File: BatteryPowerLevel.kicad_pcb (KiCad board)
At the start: 2 copper layers, 22.2 x 23.9 mm, 30 parts, among them J1 Conn_01x02_Male, SW1 SW_Push

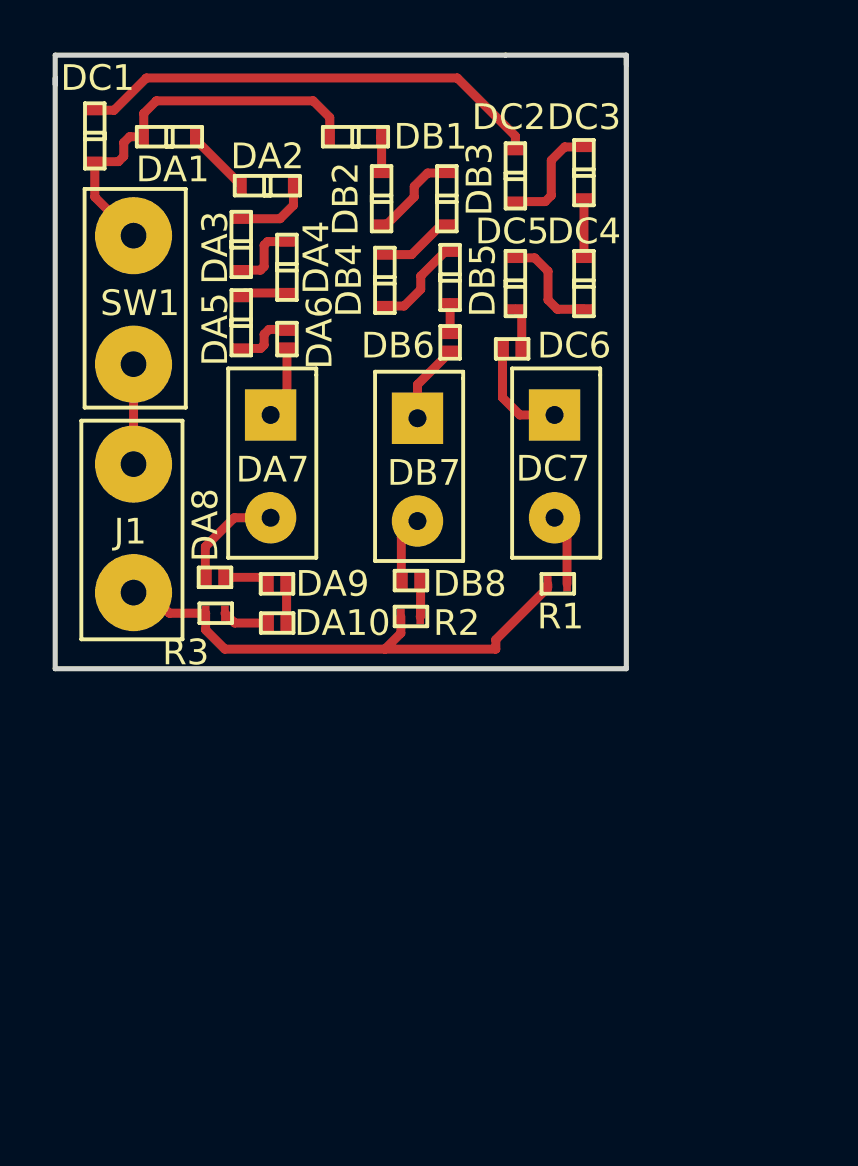
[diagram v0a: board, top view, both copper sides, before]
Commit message: Reverted
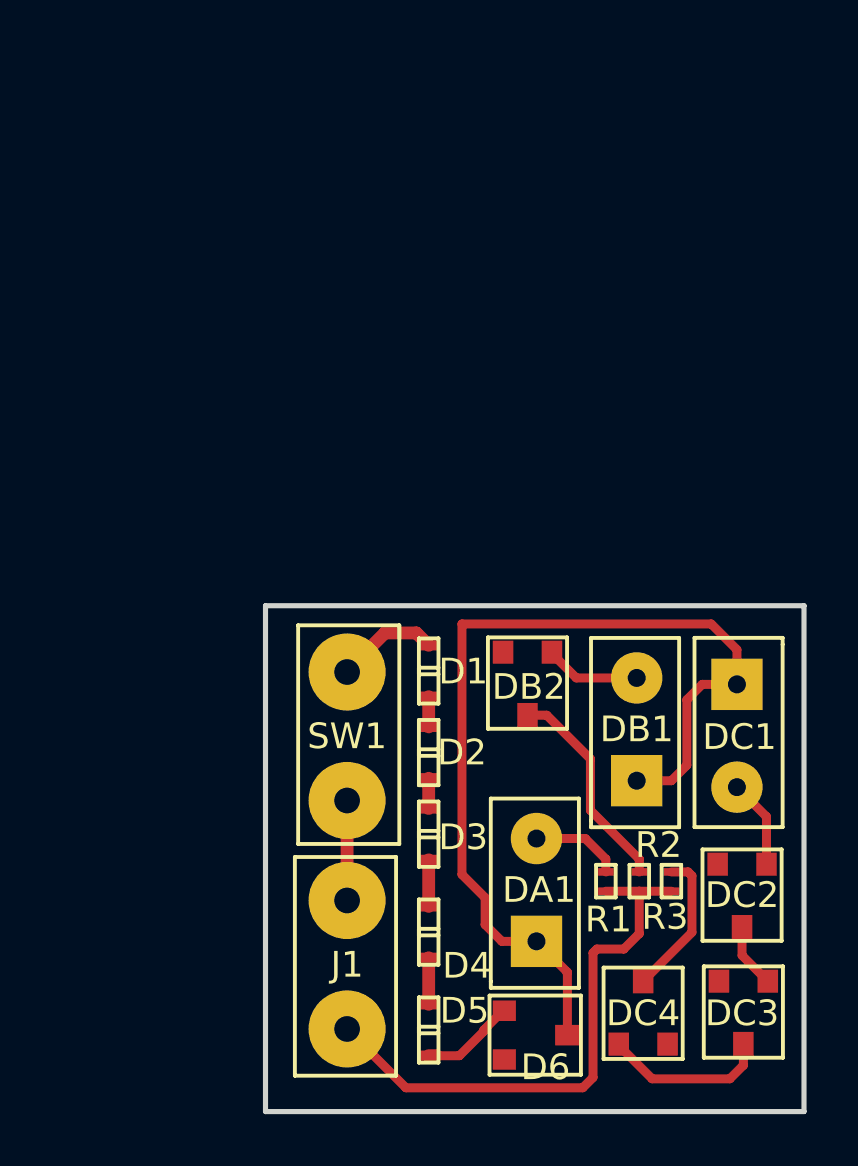
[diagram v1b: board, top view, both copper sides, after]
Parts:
- removed DA10, DA6, DA8, DA9, DB6, DB8, DC6: DIODE, Battery_Power_Level:CDSQR400B-HF (Diode 0.77V 10ohms)
- removed DA2, DA3, DA4, DA5, DB3, DB4, DB5, DC5: LED, Battery_Power_Level:LTST-C191KGKT (LED 2V)
- removed DA7, DB7, DC7: LED, Battery_Power_Level:LW514 (LED 3.2V)
- added D1: LED, Battery_Power_Level:LTST-C191KGKT (LED 2V), F.Cu at (146.1, 105.9)
- added D2: LED, Battery_Power_Level:LTST-C191KGKT (LED 2V), F.Cu at (146.1, 109.1)
- added D3: LED, Battery_Power_Level:LTST-C191KGKT (LED 2V), F.Cu at (146.1, 112.2)
- added D4: LED, Battery_Power_Level:LTST-C191KGKT (LED 2V), F.Cu at (146.1, 116.0)
- added D5: LED, Battery_Power_Level:LTST-C191KGKT (LED 2V), F.Cu at (146.1, 119.8)
- added D6: DIODE, Battery_Power_Level:MMBD914L (DIODE 0.77V), F.Cu at (148.6, 120.0)
- DA1, DB1, DC1: footprint Battery_Power_Level:LTST-C191KGKT (LED 2V) -> Battery_Power_Level:LW514 (LED 3.2V)
- DB2, DC2, DC3, DC4: value LED -> DIODE; footprint Battery_Power_Level:LTST-C191KGKT (LED 2V) -> Battery_Power_Level:MMBD914L (DIODE 0.77V)
- moved DC1 34.2 mm to (158.1, 108.4), turned to 270 degrees
- moved DA1 32.6 mm to (150.3, 114.4), turned to 90 degrees
- moved DC3 31.6 mm to (158.3, 117.5)
- moved DC4 30.1 mm to (154.4, 120.8), turned to 0 degrees
- moved DC2 27.8 mm to (158.3, 113.0)
- moved DB1 25.5 mm to (154.2, 108.2), turned to 90 degrees
- moved R3 19.9 mm to (155.6, 113.5), turned to 270 degrees
- moved J1 18.9 mm to (142.9, 117.3)
- moved SW1 18.9 mm to (142.9, 108.4)
- moved DB2 18.1 mm to (149.9, 104.7)
- moved R2 12.9 mm to (154.3, 113.5), turned to 270 degrees
- moved R1 11.1 mm to (153.0, 113.5), turned to 270 degrees
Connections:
- DA1 pad 2: Net-(DA1-Pad2) -> Net-(D6-Pad2)
- DB1 pad 2: Net-(DA1-Pad2) -> Net-(D6-Pad2)
- DB2 pad 1: Net-(DB2-Pad1) -> Net-(DB1-Pad1)
- DB2 pad 2: Net-(DB1-Pad1) -> Net-(DB2-Pad2)
- DC1 pad 2: Net-(DA1-Pad2) -> Net-(D6-Pad2)
- DC2 pad 1: Net-(DC2-Pad1) -> Net-(DC1-Pad1)
- DC2 pad 2: Net-(DC1-Pad1) -> Net-(DC2-Pad2)
- DC3 pad 1: Net-(DC3-Pad1) -> Net-(DC2-Pad2)
- DC3 pad 2: Net-(DC2-Pad1) -> Net-(DC3-Pad2)
- DC4 pad 1: Net-(DC4-Pad1) -> Net-(DC3-Pad2)
- DC4 pad 2: Net-(DC3-Pad1) -> Net-(DC4-Pad2)
- R1 pad 1: Net-(DC7-Pad1) -> Net-(DA1-Pad1)
- R2 pad 1: Net-(DB8-Pad2) -> Net-(DB2-Pad2)
- R3 pad 1: Net-(DA10-Pad2) -> Net-(DC4-Pad2)
- SW1 pad 2: Net-(DA1-Pad2) -> Net-(D1-Pad2)
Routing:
- net Net-(D6-Pad2): track 0.00 -> 37.9 mm
- net Net-(DA1-Pad2): track 15.5 -> 0.00 mm
- net Net-(DC1-Pad1): track 18.4 -> 3.48 mm
- net Net-(DB2-Pad2): track 0.00 -> 8.34 mm
- net Net-(DC3-Pad2): track 0.00 -> 6.48 mm
- net Net-(DC4-Pad2): track 0.00 -> 5.75 mm
- net Net-(DC2-Pad1): track 4.35 -> 0.00 mm
- net Net-(DC6-Pad2): track 4.20 -> 0.00 mm
- net Net-(DA7-Pad1): track 4.20 -> 0.00 mm
- net Net-(DC4-Pad1): track 4.15 -> 0.00 mm
- net Net-(D1-Pad2): track 0.00 -> 4.03 mm
- net Net-(D5-Pad1): track 0.00 -> 3.99 mm
- net Net-(DB4-Pad1): track 3.72 -> 0.00 mm
- net Net-(DB2-Pad1): track 3.61 -> 0.00 mm
- net Net-(DB6-Pad2): track 3.10 -> 0.00 mm
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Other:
- board size 22.2 x 23.9 mm -> 21 x 19.7 mm
- rule trace_min: 0.3 -> 0.2

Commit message: Revision
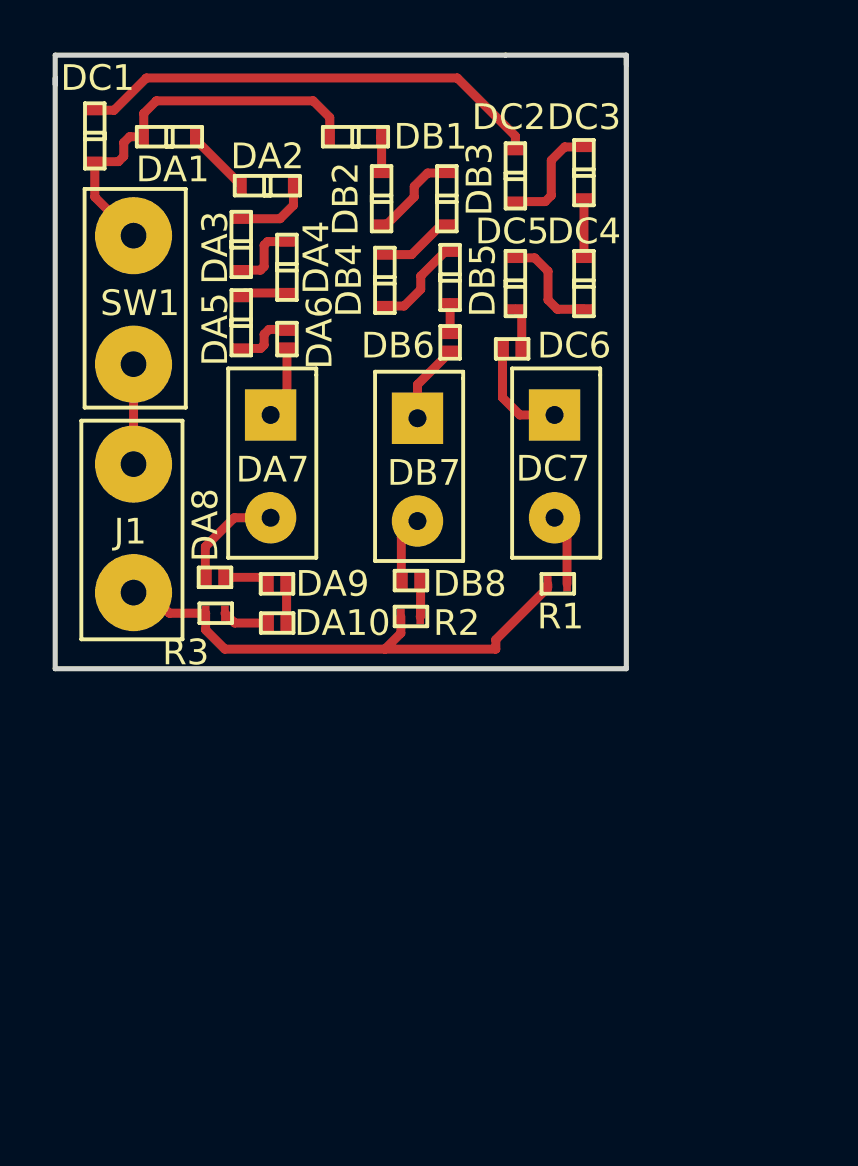
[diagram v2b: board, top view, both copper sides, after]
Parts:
- removed D1, D2, D3, D4, D5: LED, Battery_Power_Level:LTST-C191KGKT (LED 2V)
- removed D6: DIODE, Battery_Power_Level:MMBD914L (DIODE 0.77V)
- added DA10: DIODE, Battery_Power_Level:CDSQR400B-HF (Diode 0.77V 10ohms), F.Cu at (140.2, 104.0)
- added DA2: LED, Battery_Power_Level:LTST-C191KGKT (LED 2V), F.Cu at (139.8, 87.0)
- added DA3: LED, Battery_Power_Level:LTST-C191KGKT (LED 2V), F.Cu at (138.8, 89.3)
- added DA4: LED, Battery_Power_Level:LTST-C191KGKT (LED 2V), F.Cu at (140.6, 90.2)
- added DA5: LED, Battery_Power_Level:LTST-C191KGKT (LED 2V), F.Cu at (138.8, 92.3)
- added DA6: DIODE, Battery_Power_Level:CDSQR400B-HF (Diode 0.77V 10ohms), F.Cu at (140.6, 93.0)
- added DA7: LED, Battery_Power_Level:LW514 (LED 3.2V), F.Cu at (140.0, 97.9)
- added DA8: DIODE, Battery_Power_Level:CDSQR400B-HF (Diode 0.77V 10ohms), F.Cu at (137.8, 102.2)
- added DA9: DIODE, Battery_Power_Level:CDSQR400B-HF (Diode 0.77V 10ohms), F.Cu at (140.2, 102.5)
- added DB3: LED, Battery_Power_Level:LTST-C191KGKT (LED 2V), F.Cu at (146.8, 87.5)
- added DB4: LED, Battery_Power_Level:LTST-C191KGKT (LED 2V), F.Cu at (144.4, 90.7)
- added DB5: LED, Battery_Power_Level:LTST-C191KGKT (LED 2V), F.Cu at (146.9, 90.6)
- added DB6: DIODE, Battery_Power_Level:CDSQR400B-HF (Diode 0.77V 10ohms), F.Cu at (146.9, 93.1)
- added DB7: LED, Battery_Power_Level:LW514 (LED 3.2V), F.Cu at (145.7, 98.0)
- added DB8: DIODE, Battery_Power_Level:CDSQR400B-HF (Diode 0.77V 10ohms), F.Cu at (145.4, 102.4)
- added DC5: LED, Battery_Power_Level:LTST-C191KGKT (LED 2V), F.Cu at (149.5, 90.8)
- added DC6: DIODE, Battery_Power_Level:CDSQR400B-HF (Diode 0.77V 10ohms), F.Cu at (149.4, 93.3)
- added DC7: LED, Battery_Power_Level:LW514 (LED 3.2V), F.Cu at (151.0, 97.9)
- DA1, DB1, DC1: footprint Battery_Power_Level:LW514 (LED 3.2V) -> Battery_Power_Level:LTST-C191KGKT (LED 2V)
- DB2, DC2, DC3, DC4: value DIODE -> LED; footprint Battery_Power_Level:MMBD914L (DIODE 0.77V) -> Battery_Power_Level:LTST-C191KGKT (LED 2V)
- moved DC1 34.2 mm to (133.1, 85.1), turned to 0 degrees
- moved DA1 32.6 mm to (136.0, 85.1), turned to 270 degrees
- moved DC3 31.6 mm to (152.1, 86.5)
- moved DC4 30.1 mm to (152.1, 90.8), turned to 180 degrees
- moved DC2 27.8 mm to (149.5, 86.6)
- moved DB1 25.5 mm to (143.3, 85.1), turned to 270 degrees
- moved R3 19.9 mm to (138.3, 103.6), turned to 180 degrees
- moved J1 18.9 mm to (134.6, 100.3)
- moved SW1 18.9 mm to (134.6, 91.4)
- moved DB2 18.1 mm to (144.3, 87.5)
- moved R2 12.9 mm to (145.9, 103.8), turned to 180 degrees
- moved R1 11.1 mm to (151.6, 102.5), turned to 180 degrees
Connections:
- DA1 pad 2: Net-(D6-Pad2) -> Net-(DA1-Pad2)
- DB1 pad 2: Net-(D6-Pad2) -> Net-(DA1-Pad2)
- DB2 pad 1: Net-(DB1-Pad1) -> Net-(DB2-Pad1)
- DB2 pad 2: Net-(DB2-Pad2) -> Net-(DB1-Pad1)
- DC1 pad 2: Net-(D6-Pad2) -> Net-(DA1-Pad2)
- DC2 pad 1: Net-(DC1-Pad1) -> Net-(DC2-Pad1)
- DC2 pad 2: Net-(DC2-Pad2) -> Net-(DC1-Pad1)
- DC3 pad 1: Net-(DC2-Pad2) -> Net-(DC3-Pad1)
- DC3 pad 2: Net-(DC3-Pad2) -> Net-(DC2-Pad1)
- DC4 pad 1: Net-(DC3-Pad2) -> Net-(DC4-Pad1)
- DC4 pad 2: Net-(DC4-Pad2) -> Net-(DC3-Pad1)
- R1 pad 1: Net-(DA1-Pad1) -> Net-(DC7-Pad1)
- R2 pad 1: Net-(DB2-Pad2) -> Net-(DB8-Pad2)
- R3 pad 1: Net-(DC4-Pad2) -> Net-(DA10-Pad2)
- SW1 pad 2: Net-(D1-Pad2) -> Net-(DA1-Pad2)
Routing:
- net Net-(D6-Pad2): track 37.9 -> 0.00 mm
- net Net-(DA1-Pad2): track 0.00 -> 15.5 mm
- net Net-(DC1-Pad1): track 3.48 -> 18.4 mm
- net Net-(DB2-Pad2): track 8.34 -> 0.00 mm
- net Net-(DC3-Pad2): track 6.48 -> 0.00 mm
- net Net-(DC4-Pad2): track 5.75 -> 0.00 mm
- net Net-(DC2-Pad1): track 0.00 -> 4.35 mm
- net Net-(DC6-Pad2): track 0.00 -> 4.20 mm
- net Net-(DA7-Pad1): track 0.00 -> 4.20 mm
- net Net-(DC4-Pad1): track 0.00 -> 4.15 mm
- net Net-(D1-Pad2): track 4.03 -> 0.00 mm
- net Net-(D5-Pad1): track 3.99 -> 0.00 mm
- net Net-(DB4-Pad1): track 0.00 -> 3.72 mm
- net Net-(DB2-Pad1): track 0.00 -> 3.61 mm
- net Net-(DB6-Pad2): track 0.00 -> 3.10 mm
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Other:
- board size 21 x 19.7 mm -> 22.2 x 23.9 mm
- rule trace_min: 0.2 -> 0.3
